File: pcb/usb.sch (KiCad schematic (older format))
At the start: 9 parts, among them J600 USB_B_Micro, U600 USBLC6-2SC6

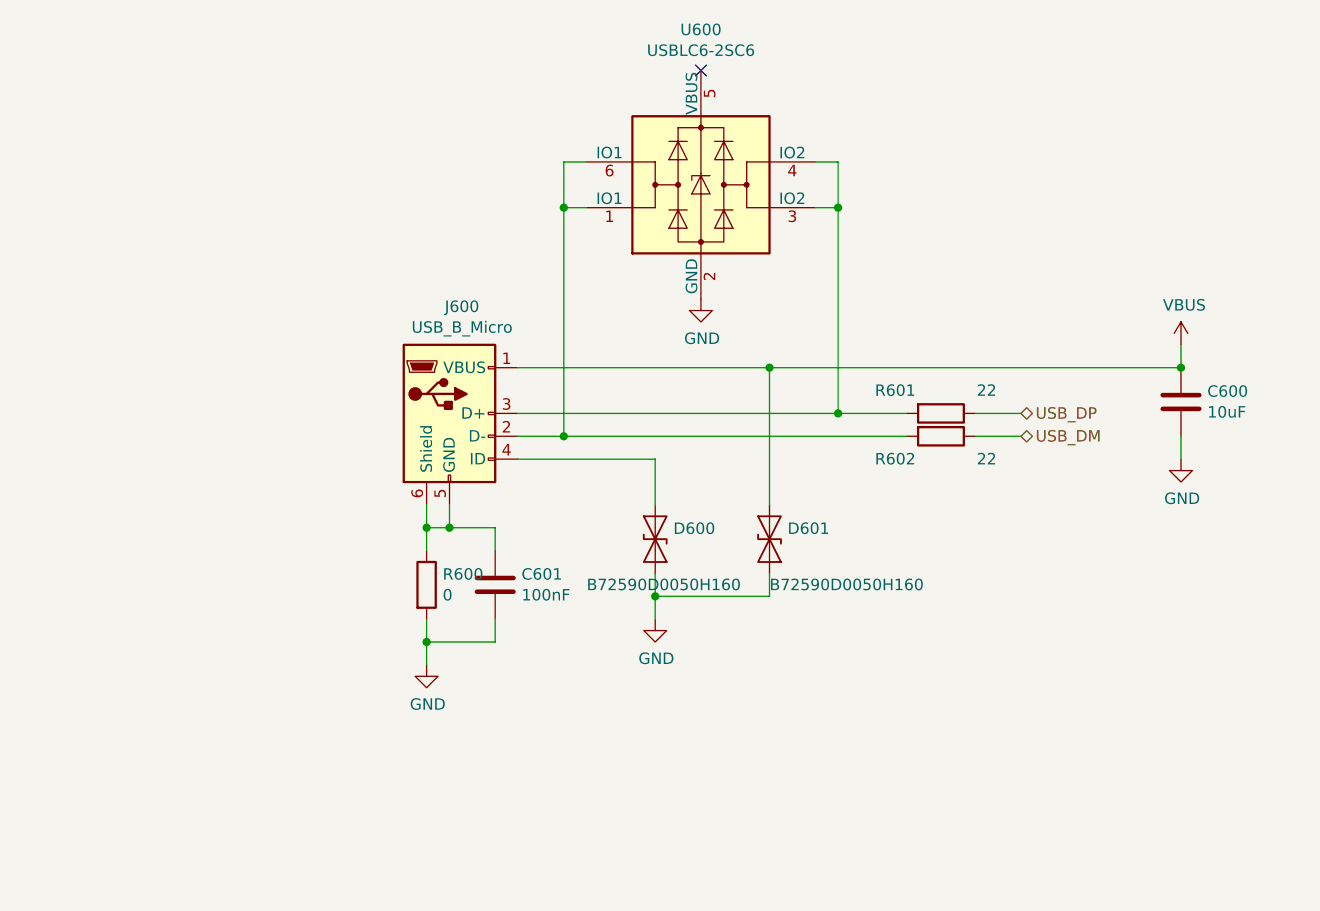
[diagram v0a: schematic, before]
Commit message: pcb: working on sch
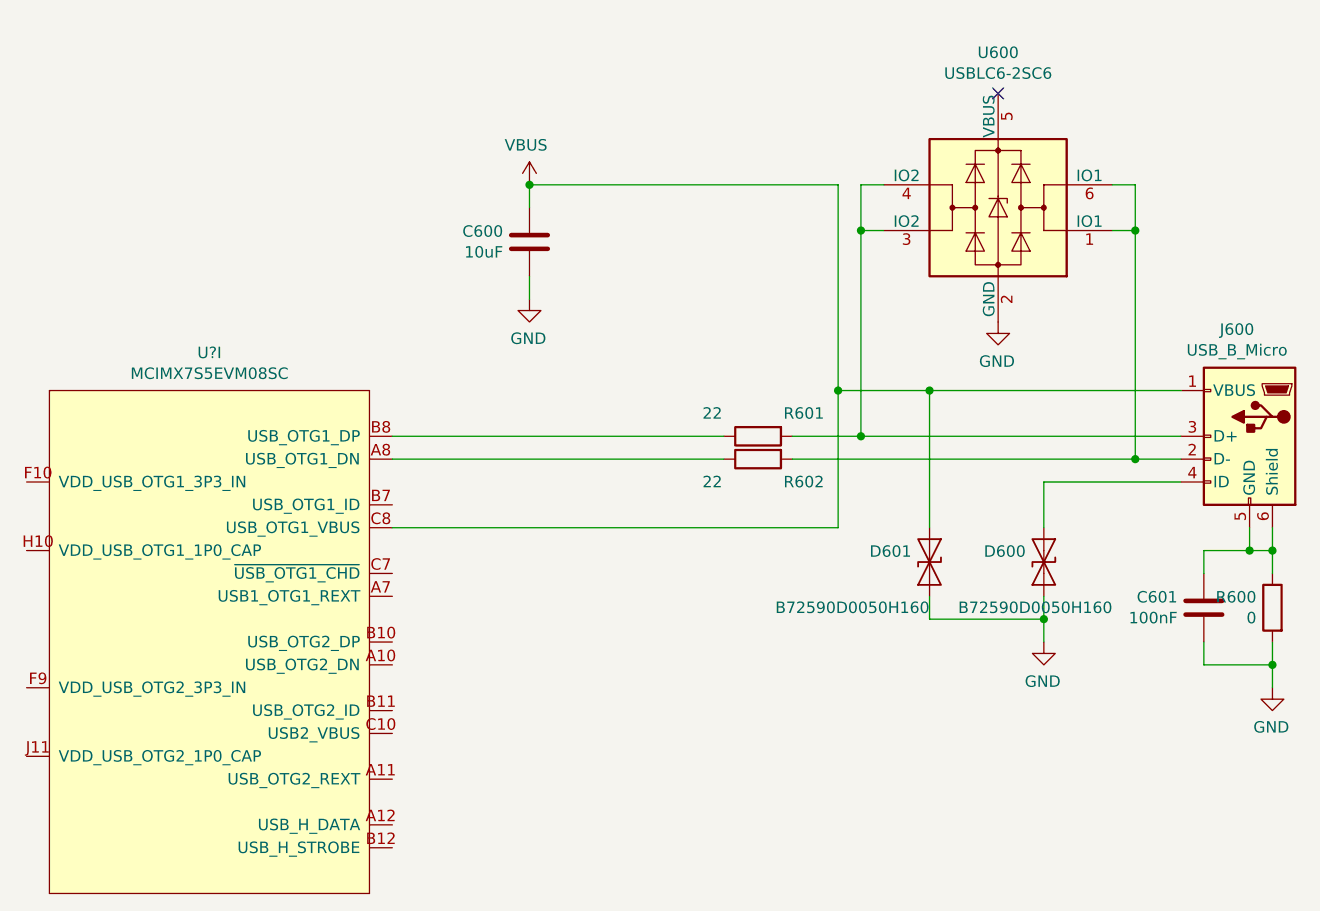
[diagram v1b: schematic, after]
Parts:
- added U?: MCIMX7S5EVM08SC, footprints:BGA-541_25x25_19.0x19.0mm, symbol symbols:MCIMX7S5EVM08SC
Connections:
- net VBUS: now also U?.C8 (USB_OTG1_VBUS)
- net USB_DM: no longer names the net of R602.1
- net USB_DM: now also U?.A8 (USB_OTG1_DN)
- net USB_DP: no longer names the net of R601.1
- net USB_DP: now also U?.B8 (USB_OTG1_DP)
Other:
- moved on the sheet: C600, C601, D600, D601, J600, R600, R601, R602, U600
